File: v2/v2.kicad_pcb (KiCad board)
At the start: 2 copper layers, 9.7 x 8.4 mm, 105 parts, among them J1 Conn_01x04_Pin, J2 Conn_01x04_Pin, J3 Conn_01x04_Pin, SW1 SW_Push, SW10 SW_Push, SW11 SW_Push, SW12 SW_Push, SW13 SW_Push, SW14 SW_Push, SW15 SW_Push, SW16 SW_Push, SW17 SW_Push, SW18 SW_Push, SW19 SW_Push, SW2 SW_Push, SW20 SW_Push, SW21 SW_Push, SW22 SW_Push, SW23 SW_Push, SW24 SW_Push, SW25 SW_Push, SW26 SW_Push, SW27 SW_Push, SW28 SW_Push, SW29 SW_Push, SW3 SW_Push, SW30 SW_Push, SW31 SW_Push, SW32 SW_Push, SW33 RotaryEncoder_Switch, SW4 SW_Push, SW5 SW_Push, SW6 SW_Push, SW7 SW_Push, SW8 SW_Push, SW9 SW_Push, U1 Pico, U2 Pico

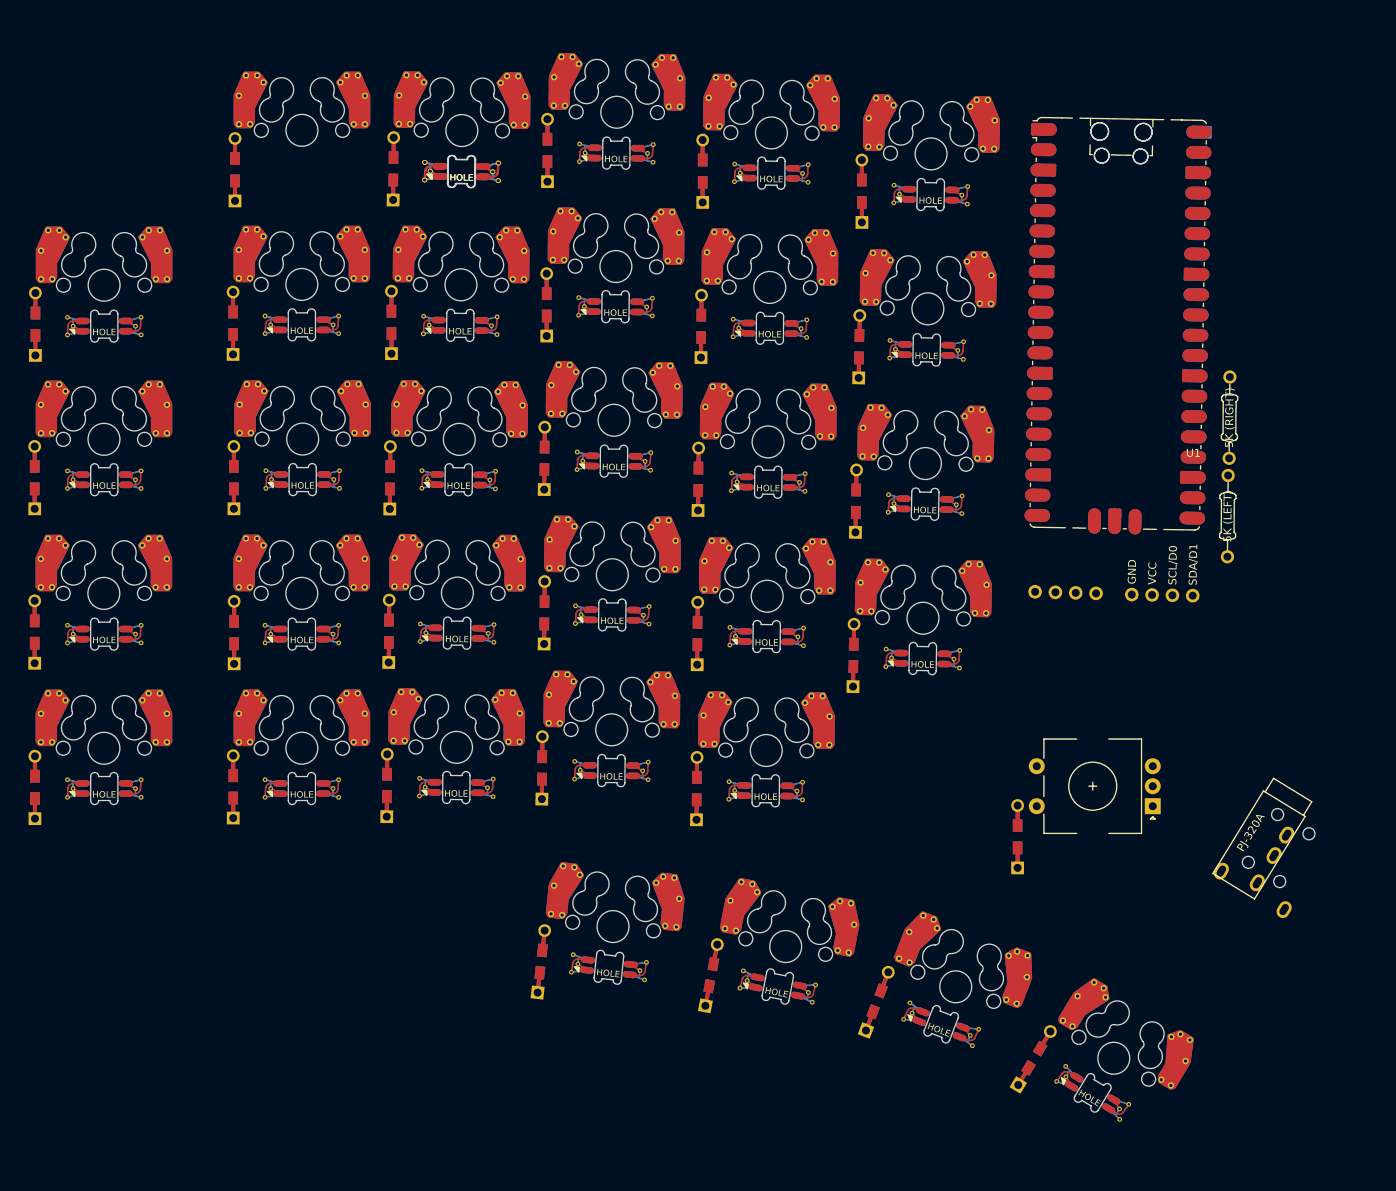
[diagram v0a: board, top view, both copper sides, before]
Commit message: started running traces
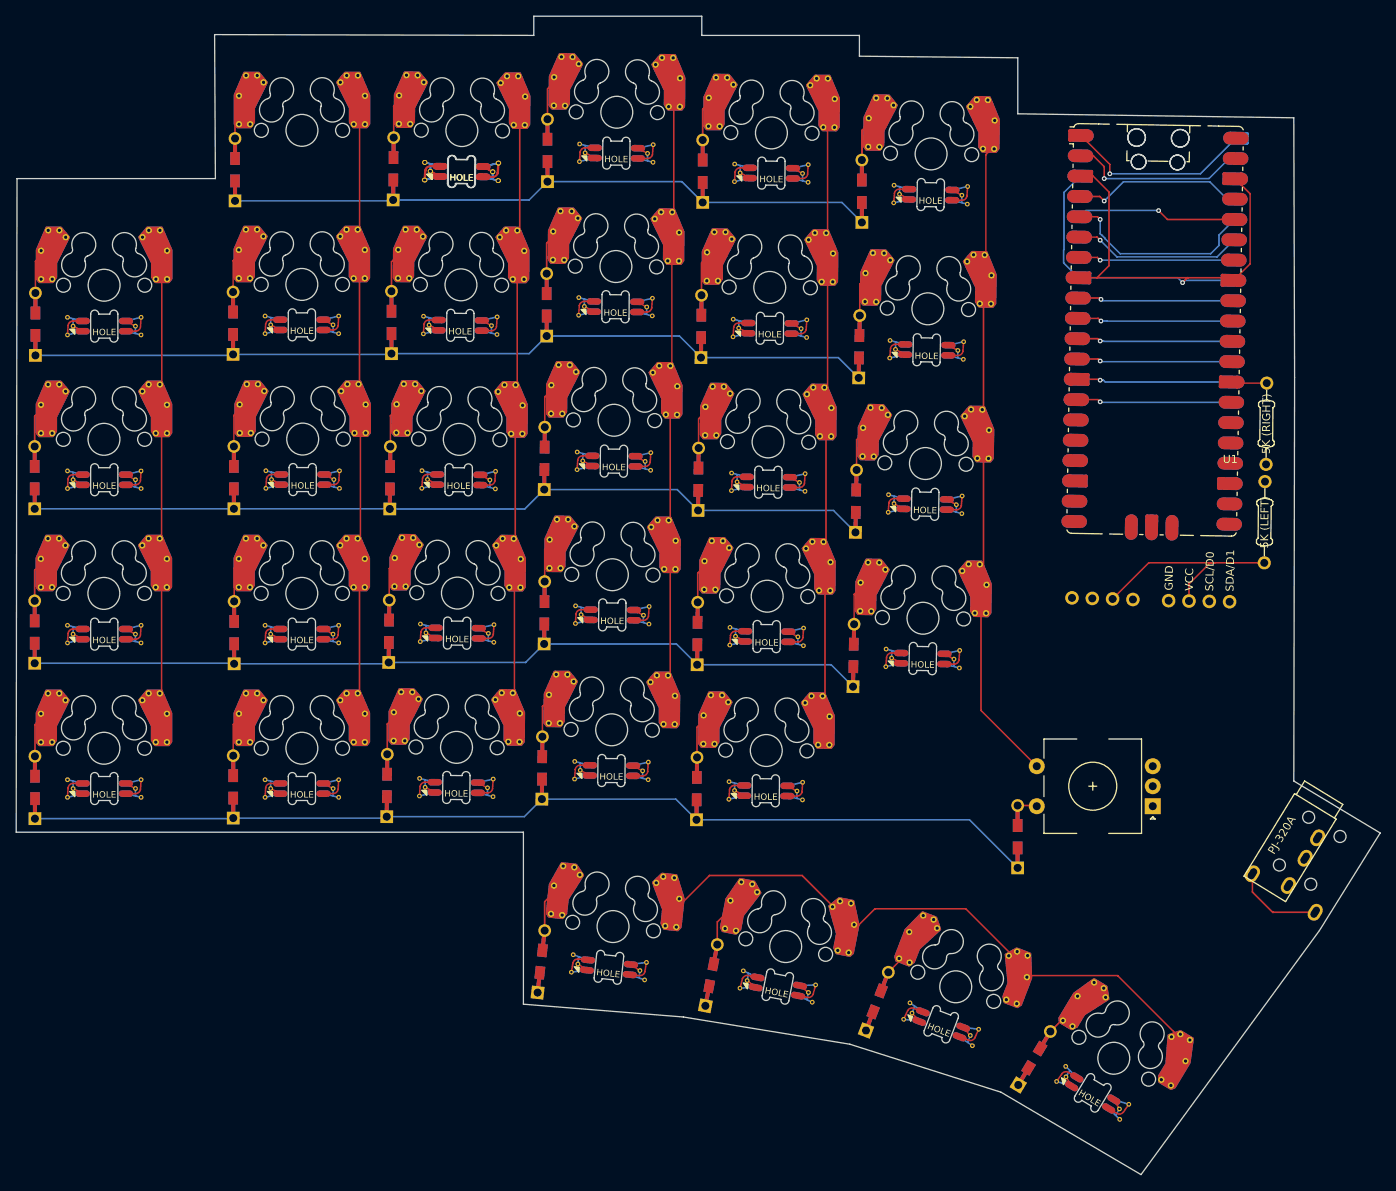
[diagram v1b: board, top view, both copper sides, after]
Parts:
- moved U1 4.67 mm to (257.7, 122.0)
- moved U2 4.67 mm to (257.7, 122.0)
- moved J2 4.67 mm to (259.4, 155.9)
- moved J1 4.67 mm to (254.9, 155.7)
- moved R3 4.67 mm to (271.4, 146.1)
- moved R4 4.67 mm to (271.6, 133.7)
- moved J3 3.90 mm to (279.7, 182.8)
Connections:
- D2 pad 1: Net-(D2-K) -> Row 1
- D3 pad 1: Net-(D2-K) -> Row 1
- D4 pad 1: Net-(D2-K) -> Row 1
- D5 pad 1: Net-(D2-K) -> Row 1
- D6 pad 1: Net-(D2-K) -> Row 1
- D7 pad 1: Net-(D2-K) -> Row 1
- U1 pad 31: unconnected-(U1-GPIO26_ADC0-Pad31) -> ENC B
- U1 pad 32: unconnected-(U1-GPIO27_ADC1-Pad32) -> ENC A
- U1 pad 36: unconnected-(U1-3V3-Pad36) -> +3.3V
- U2 pad 24: unconnected-(U2-GPIO18-Pad24) -> SERIAL B
- U2 pad 25: unconnected-(U2-GPIO19-Pad25) -> SERIAL A
- U2 pad 31: unconnected-(U2-GPIO26_ADC0-Pad31) -> ENC B
- U2 pad 32: unconnected-(U2-GPIO27_ADC1-Pad32) -> ENC A
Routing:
- net Row 5: track 0.00 -> 146.9 mm, vias 0 -> 1
- net Row 2: track 0.00 -> 125.6 mm, vias 0 -> 1
- net Row 3: track 0.00 -> 125.3 mm, vias 0 -> 1
- net Row 4: track 0.00 -> 125.1 mm, vias 0 -> 1
- net Col 7: track 0.00 -> 104.7 mm, vias 0 -> 1
- net Col 4: track 0.00 -> 102.4 mm, vias 0 -> 1
- net Col 6: track 0.00 -> 101.8 mm, vias 0 -> 1
- net Row 1: track 0.00 -> 101.0 mm, vias 0 -> 1
- net GND: track 0.00 -> 100.2 mm, vias 0 -> 1
- net Col 2: track 0.00 -> 99.8 mm, vias 0 -> 1
- net Col 5: track 0.00 -> 98.8 mm, vias 0 -> 1
- net Col 3: track 0.00 -> 97.3 mm, vias 0 -> 1
- net Col 1: track 0.00 -> 81.8 mm, vias 0 -> 1
- net +3.3V: track 0.00 -> 47.4 mm, vias 0 -> 1
- net Net-(D6-A): track 0.00 -> 13.8 mm
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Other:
- board size 9.7 x 8.4 mm -> 170.5 x 144.8 mm
